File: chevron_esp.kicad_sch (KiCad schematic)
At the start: 21 parts, among them J1 282837-4, J2 MTSW-101-09-G-S-104x4, K1 SRD-05VDC-SL-C, K2 SRD-05VDC-SL-C, K3 SRD-05VDC-SL-C, P1 282837-2, Q1 PN2222A, Q2 PN2222A, Q3 PN2222A, SW1 1825057-2, U1 ESP32-DEVKIT-V1, U2 RA-02_LORA

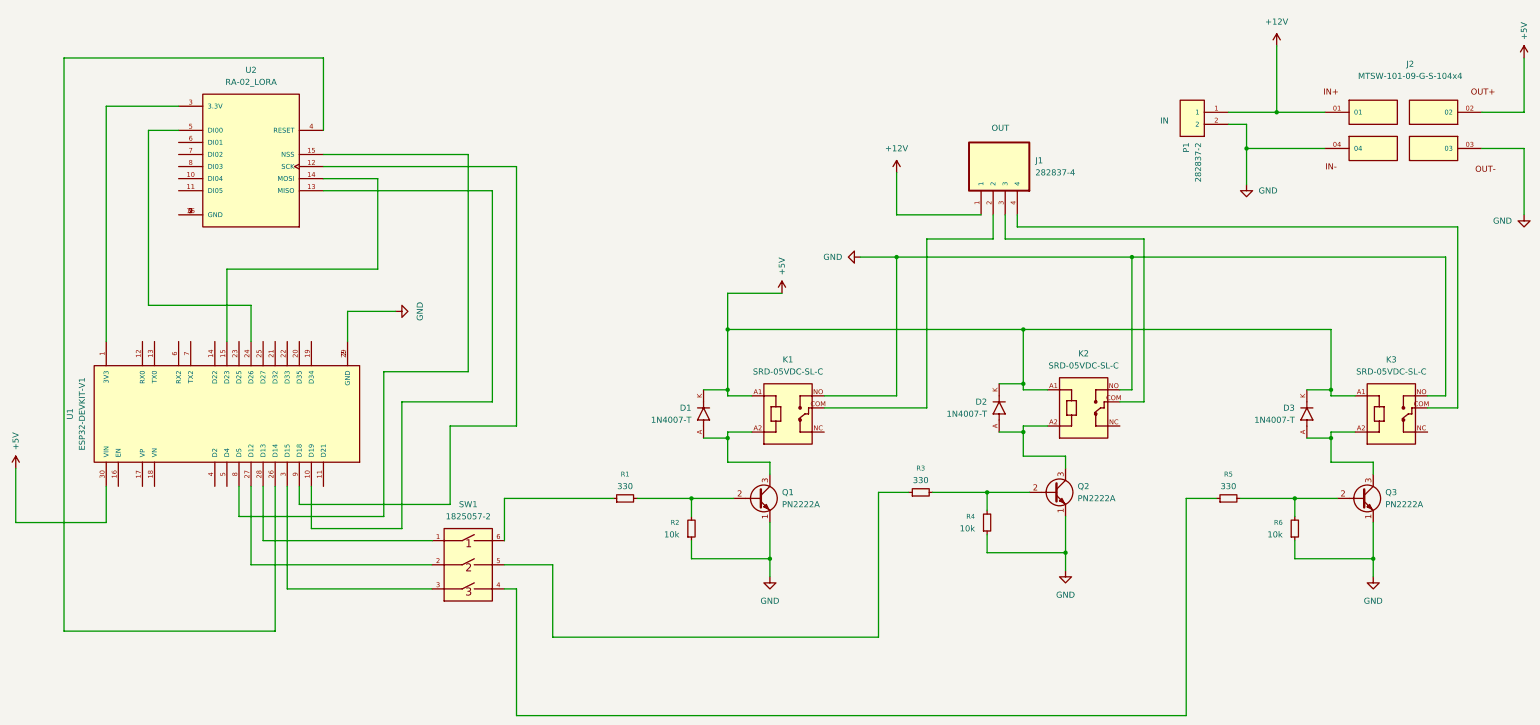
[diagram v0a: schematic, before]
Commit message: v1 ok
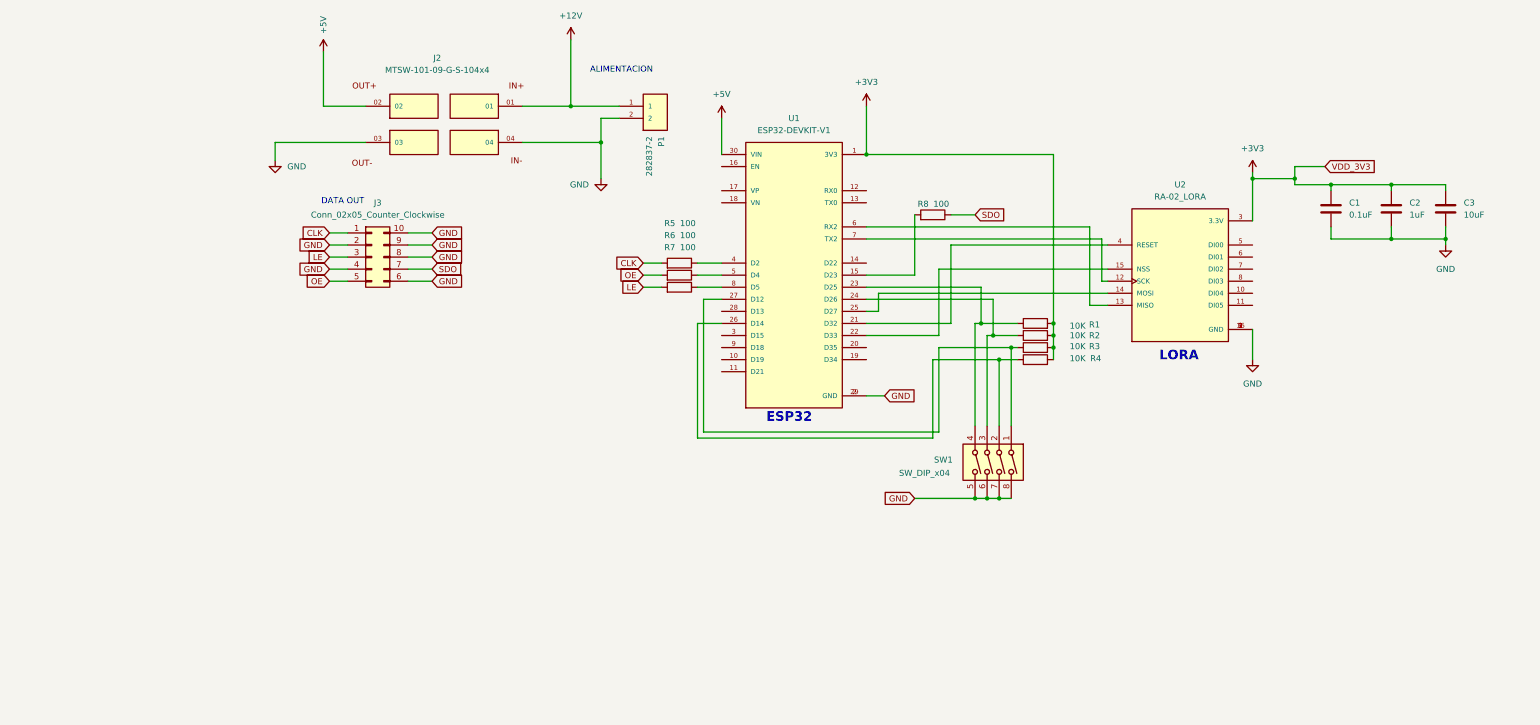
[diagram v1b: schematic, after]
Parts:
- removed D1, D2, D3: 1N4007-T, 1N4007-T:DIOAD780W78L463D236, symbol 1N4007-T:1N4007-T
- removed J1: 282837-4, 282837-4:TE_282837-4, symbol 282837-4:282837-4
- removed K1, K2, K3: SRD-05VDC-SL-C, SRD-05VDC-SL-C:RELAY_SRD-05VDC-SL-C, symbol SRD-05VDC-SL-C:SRD-05VDC-SL-C
- removed Q1, Q2, Q3: PN2222A, Package_TO_SOT_THT:TO-92_Inline, symbol Transistor_BJT:PN2222A
- removed R1, R3, R5: 330, Resistor_SMD:R_1206_3216Metric, symbol Device:R_Small
- removed R2, R4, R6: 10k, Resistor_SMD:R_1206_3216Metric, symbol Device:R_Small
- removed SW1: 1825057-2, 1825057-2:DIP810W60P254L1010H480Q6, symbol 1825057-2:1825057-2
- added C1: 0.1uF, Capacitor_SMD:C_0603_1608Metric_Pad1.08x0.95mm_HandSolder, symbol Device:C
- added C2: 1uF, Capacitor_SMD:C_1206_3216Metric_Pad1.33x1.80mm_HandSolder, symbol Device:C
- added C3: 10uF, Capacitor_SMD:C_0805_2012Metric_Pad1.18x1.45mm_HandSolder, symbol Device:C
- added J3: Conn_02x05_Counter_Clockwise, Connector_IDC:IDC-Header_2x05_P2.54mm_Vertical, symbol Connector_Generic:Conn_02x05_Counter_Clockwise
- added R1, R2, R3, R4: 10K, Resistor_SMD:R_1206_3216Metric_Pad1.30x1.75mm_HandSolder, symbol Device:R
- added R5, R6, R7, R8: 100, Resistor_SMD:R_1206_3216Metric_Pad1.30x1.75mm_HandSolder, symbol Device:R
- added SW1: SW_DIP_x04, Button_Switch_THT:SW_DIP_SPSTx04_Slide_6.7x11.72mm_W7.62mm_P2.54mm_LowProfile, symbol Switch:SW_DIP_x04
- P1: footprint 282837-2:TE_282837-2 -> Connector_PinHeader_2.54mm:PinHeader_1x02_P2.54mm_Vertical; DESCRIPTION TERMINAL BLOCK 3.5MM 2POS PCB -> (none)
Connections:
- net GND: now also U2.1 (GND), U2.16 (GND), U2.2 (GND), U2.9 (GND), C1.2, C2.2, C3.2, J3.10 (Pin_10), J3.2 (Pin_2), J3.4 (Pin_4), J3.6 (Pin_6), J3.8 (Pin_8), J3.9 (Pin_9), SW1.5, SW1.6, SW1.7, SW1.8
- net +3V3: now reaches U1.1 (3V3), U2.3 (3.3V)
- net +3V3: now also C1.1, C2.1, C3.1, R1.2, R2.2, R3.2, R4.2
- net at U1.10 (D19): no longer U2.13 (MISO)
- net at U1.15 (D23): now also R8.2; no longer U2.14 (MOSI)
- net at U1.21 (D32): now also U2.4 (RESET)
- net at U1.22 (D33): now also U2.15 (NSS)
- net at U1.23 (D25): now also R1.1, SW1.4
- net at U1.24 (D26): now also R2.1, SW1.3; no longer U2.5 (DI00)
- net at U1.25 (D27): now also U2.14 (MOSI)
- net at U1.26 (D14): now also R4.1, SW1.2; no longer U2.4 (RESET)
- net at U1.27 (D12): now also R3.1, SW1.1
- net at U1.4 (D2): now also R5.1
- net at U1.5 (D4): now also R6.1
- net at U1.6 (RX2): now also U2.13 (MISO)
- net at U1.7 (TX2): now also U2.12 (SCK)
- net at U1.8 (D5): now also R7.1; no longer U2.15 (NSS)
- net at U1.9 (D18): no longer U2.12 (SCK)
- new net CLK: J3.1 (Pin_1), R5.2
- new net LE: J3.3 (Pin_3), R7.2
- new net OE: J3.5 (Pin_5), R6.2
- new net SDO: J3.7 (Pin_7), R8.1
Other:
- note added: "ALIMENTACION"
- note added: "DATA OUT"
- note added: "ESP32"
- note added: "LORA"
- note removed: "IN"
- note removed: "OUT"
- moved on the sheet: J2, P1
